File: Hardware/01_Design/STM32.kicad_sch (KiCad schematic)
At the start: 19 parts, among them J2 Conn_01x04, SW1 EN, U3 STM32F103C8T6, Y1 8MHz_3225

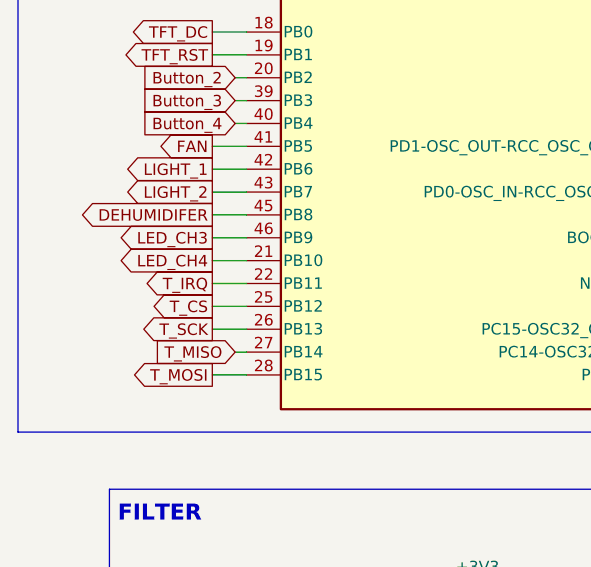
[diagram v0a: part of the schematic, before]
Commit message: Placement component
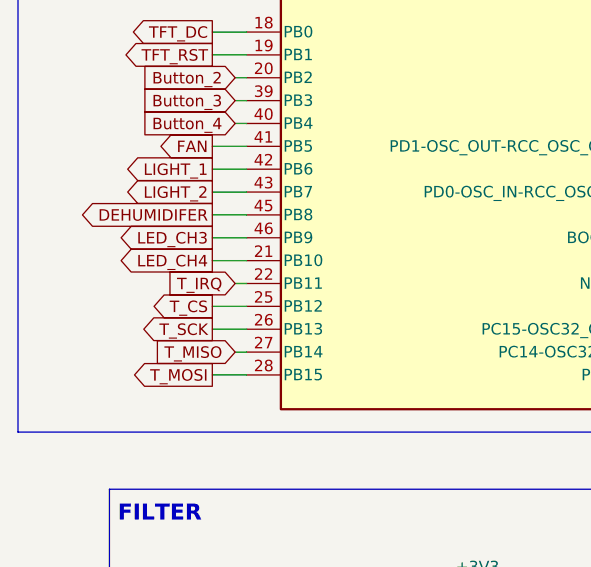
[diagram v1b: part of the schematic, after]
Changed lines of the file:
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@@
 	(wire
 		(pts
-			(xy 49.53 100.33) (xy 53.34 100.33)
+			(xy 52.07 100.33) (xy 53.34 100.33)
 		)
 		(stroke
@@
 	)
 	(global_label "T_IRQ"
-		(shape output)
-		(at 49.53 100.33 180)
+		(shape input)
+		(at 52.07 100.33 180)
 		(fields_autoplaced yes)
 		(effects
@@
 		)
 		(property "Intersheetrefs" "${INTERSHEET_REFS}"
-			(at 41.4043 100.33 0)
+			(at 43.9443 100.33 0)
 			(hide yes)
 			(show_name no)
